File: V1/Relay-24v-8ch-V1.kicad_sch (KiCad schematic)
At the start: 49 parts, among them J1 Conn_01x09, J3 OUT1, J3 OUT2, J3 OUT3, J3 OUT4, J3 OUT5, J3 OUT6, J3 OUT7, J3 OUT8, K1 G5PZ-1A

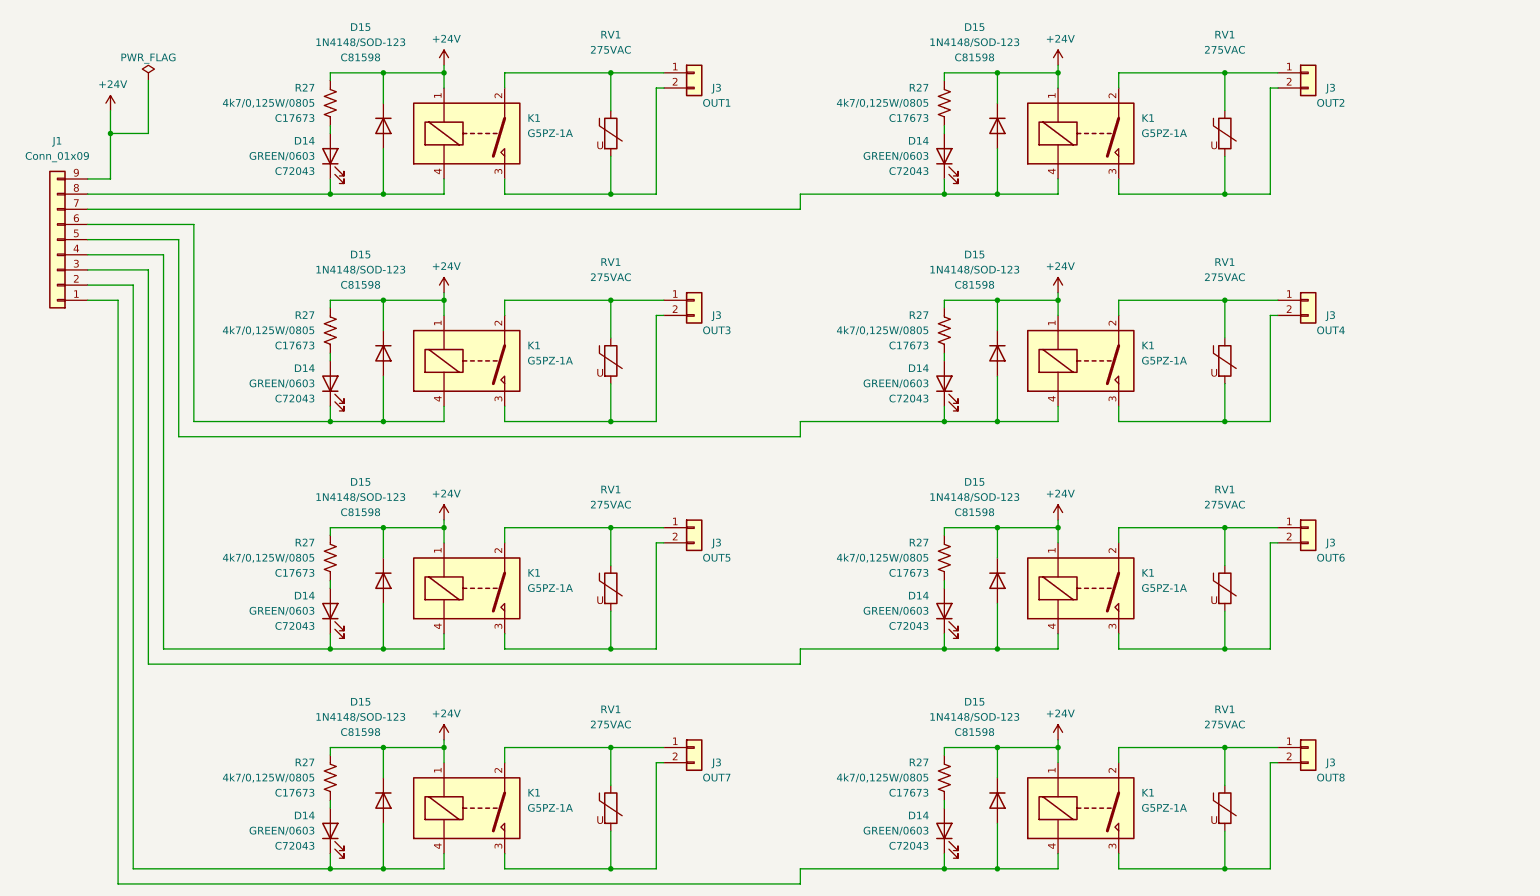
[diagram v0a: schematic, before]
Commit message: Cleanup
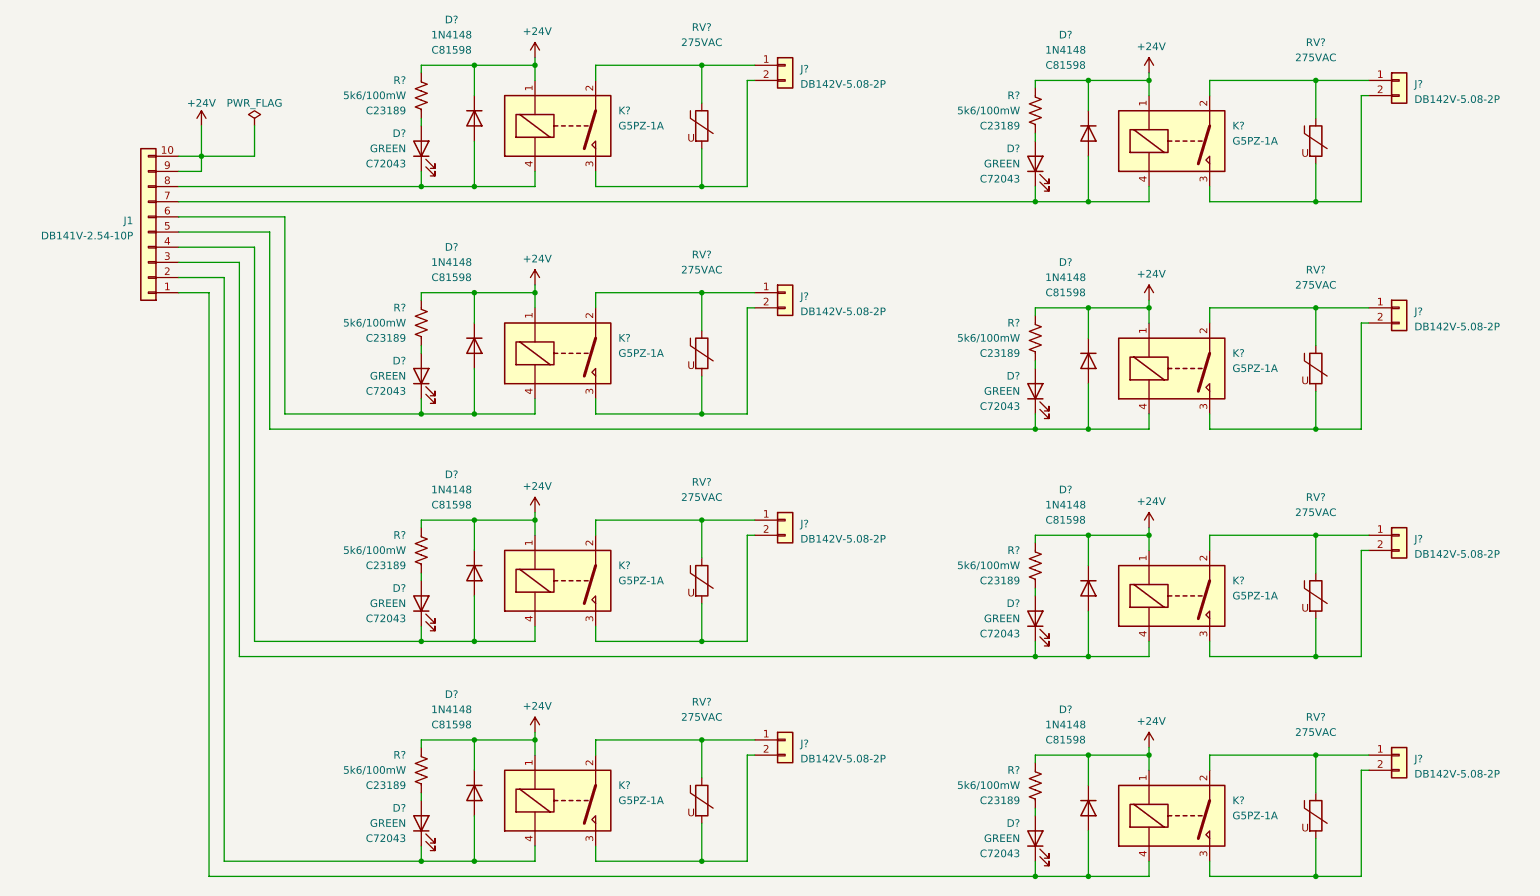
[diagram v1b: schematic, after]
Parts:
- D? (x8): renamed from D14; value GREEN/0603 -> GREEN; Case 0603 -> (none); Package (none) -> 0603/1608
- D? (x8): renamed from D15; value 1N4148/SOD-123 -> 1N4148; Case SOD-123 -> (none); Package (none) -> SOD-123
- J1: value Conn_01x09 -> DB141V-2.54-10P; footprint Tales:TerminalBlock_DG141V-2.54-9P_1x09_P2.54mm_Vertical -> Tales:TerminalBlock_Dibo_DB141V-2.54-10P_1x10_P2.54mm_Vertical; symbol Connector_Generic:Conn_01x09 -> Connector_Generic:Conn_01x10; LCSC Part # C2898751 -> C2898752; Mfr PN DB141V-2.54-9P -> DB141V-2.54-10P; Vendor PN C2898751 -> C2898752
- J?: renamed from J3; value OUT7 -> DB142V-5.08-2P; footprint Tales:TerminalBlock_Phoenix_MKDS-3-2-5.08_1x02_P5.08mm_Horizontal -> Tales:TerminalBlock_Dibo_DB142V-5.08-2P_1x02_P5.08mm_Vertical; JLCPCB BOM 0 -> 1; LCSC Part # (none) -> C2898699; Mfr Metaltex -> DIBO; Mfr PN BR902V -> DB142V-5.08-2P; Vendor Eletropeças -> JLCPCB; Vendor PN 29273 -> C2898699
- J?: renamed from J3; value OUT4 -> DB142V-5.08-2P; footprint Tales:TerminalBlock_Phoenix_MKDS-3-2-5.08_1x02_P5.08mm_Horizontal -> Tales:TerminalBlock_Dibo_DB142V-5.08-2P_1x02_P5.08mm_Vertical; JLCPCB BOM 0 -> 1; LCSC Part # (none) -> C2898699; Mfr Metaltex -> DIBO; Mfr PN BR902V -> DB142V-5.08-2P; Vendor Eletropeças -> JLCPCB; Vendor PN 29273 -> C2898699
- J?: renamed from J3; value OUT2 -> DB142V-5.08-2P; footprint Tales:TerminalBlock_Phoenix_MKDS-3-2-5.08_1x02_P5.08mm_Horizontal -> Tales:TerminalBlock_Dibo_DB142V-5.08-2P_1x02_P5.08mm_Vertical; JLCPCB BOM 0 -> 1; LCSC Part # (none) -> C2898699; Mfr Metaltex -> DIBO; Mfr PN BR902V -> DB142V-5.08-2P; Vendor Eletropeças -> JLCPCB; Vendor PN 29273 -> C2898699
- J?: renamed from J3; value OUT1 -> DB142V-5.08-2P; footprint Tales:TerminalBlock_Phoenix_MKDS-3-2-5.08_1x02_P5.08mm_Horizontal -> Tales:TerminalBlock_Dibo_DB142V-5.08-2P_1x02_P5.08mm_Vertical; JLCPCB BOM 0 -> 1; LCSC Part # (none) -> C2898699; Mfr Metaltex -> DIBO; Mfr PN BR902V -> DB142V-5.08-2P; Vendor Eletropeças -> JLCPCB; Vendor PN 29273 -> C2898699
- J?: renamed from J3; value OUT3 -> DB142V-5.08-2P; footprint Tales:TerminalBlock_Phoenix_MKDS-3-2-5.08_1x02_P5.08mm_Horizontal -> Tales:TerminalBlock_Dibo_DB142V-5.08-2P_1x02_P5.08mm_Vertical; JLCPCB BOM 0 -> 1; LCSC Part # (none) -> C2898699; Mfr Metaltex -> DIBO; Mfr PN BR902V -> DB142V-5.08-2P; Vendor Eletropeças -> JLCPCB; Vendor PN 29273 -> C2898699
- J?: renamed from J3; value OUT8 -> DB142V-5.08-2P; footprint Tales:TerminalBlock_Phoenix_MKDS-3-2-5.08_1x02_P5.08mm_Horizontal -> Tales:TerminalBlock_Dibo_DB142V-5.08-2P_1x02_P5.08mm_Vertical; JLCPCB BOM 0 -> 1; LCSC Part # (none) -> C2898699; Mfr Metaltex -> DIBO; Mfr PN BR902V -> DB142V-5.08-2P; Vendor Eletropeças -> JLCPCB; Vendor PN 29273 -> C2898699
- J?: renamed from J3; value OUT6 -> DB142V-5.08-2P; footprint Tales:TerminalBlock_Phoenix_MKDS-3-2-5.08_1x02_P5.08mm_Horizontal -> Tales:TerminalBlock_Dibo_DB142V-5.08-2P_1x02_P5.08mm_Vertical; JLCPCB BOM 0 -> 1; LCSC Part # (none) -> C2898699; Mfr Metaltex -> DIBO; Mfr PN BR902V -> DB142V-5.08-2P; Vendor Eletropeças -> JLCPCB; Vendor PN 29273 -> C2898699
- J?: renamed from J3; value OUT5 -> DB142V-5.08-2P; footprint Tales:TerminalBlock_Phoenix_MKDS-3-2-5.08_1x02_P5.08mm_Horizontal -> Tales:TerminalBlock_Dibo_DB142V-5.08-2P_1x02_P5.08mm_Vertical; JLCPCB BOM 0 -> 1; LCSC Part # (none) -> C2898699; Mfr Metaltex -> DIBO; Mfr PN BR902V -> DB142V-5.08-2P; Vendor Eletropeças -> JLCPCB; Vendor PN 29273 -> C2898699
- K? (x8): renamed from K1; footprint Tales:Relay_SPST_Omron-G5PZ-1A -> Tales:Relay_SPST_Omron_G5PZ-1A
- R? (x8): renamed from R27; value 4k7/0,125W/0805 -> 5k6/100mW; footprint Tales:R_0805_2012Metric -> Tales:R_0603_1608Metric; Case 0805/2012 -> (none); LCSC Part # C17673 -> C23189; Mfr PN 0805W8F4701T5E -> 0603WAF5601T5E; Package (none) -> 0603/1608; Vendor PN C17673 -> C23189
- RV? (x8): renamed from RV1; footprint Tales:RV_Disc_D12mm_W3.9mm_P7.5mm -> Tales:RV_Disc_D9.50mm_W3.6mm_P5.08mm; JLCPCB BOM 0 -> 1; LCSC Part # (none) -> C2761646; Mfr Yageo -> Dersonic; Mfr PN 431KD10 -> RM07D431KC1IE100; Package (none) -> 9.5x5.08mm; Vendor Mouser -> JLCPCB; Vendor PN 603-431KD10 -> C2761646
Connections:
- net +24V: now also J1.10 (Pin_10)
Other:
- moved on the sheet: D?, J?, K?, R?, RV?
